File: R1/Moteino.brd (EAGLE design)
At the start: 33.3 x 23.1 mm, 21 parts, among them IC3 MCP1703CB, X1 16 MHz

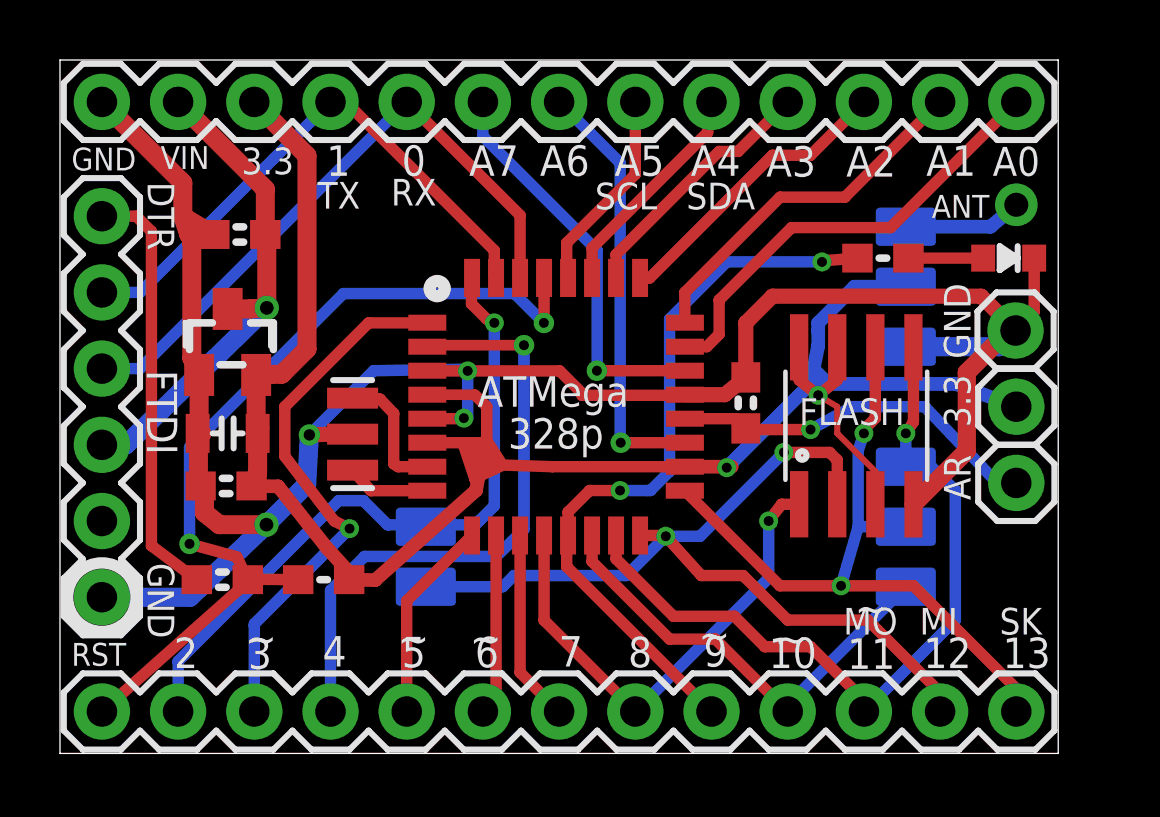
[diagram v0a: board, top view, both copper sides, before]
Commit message: R2 Update
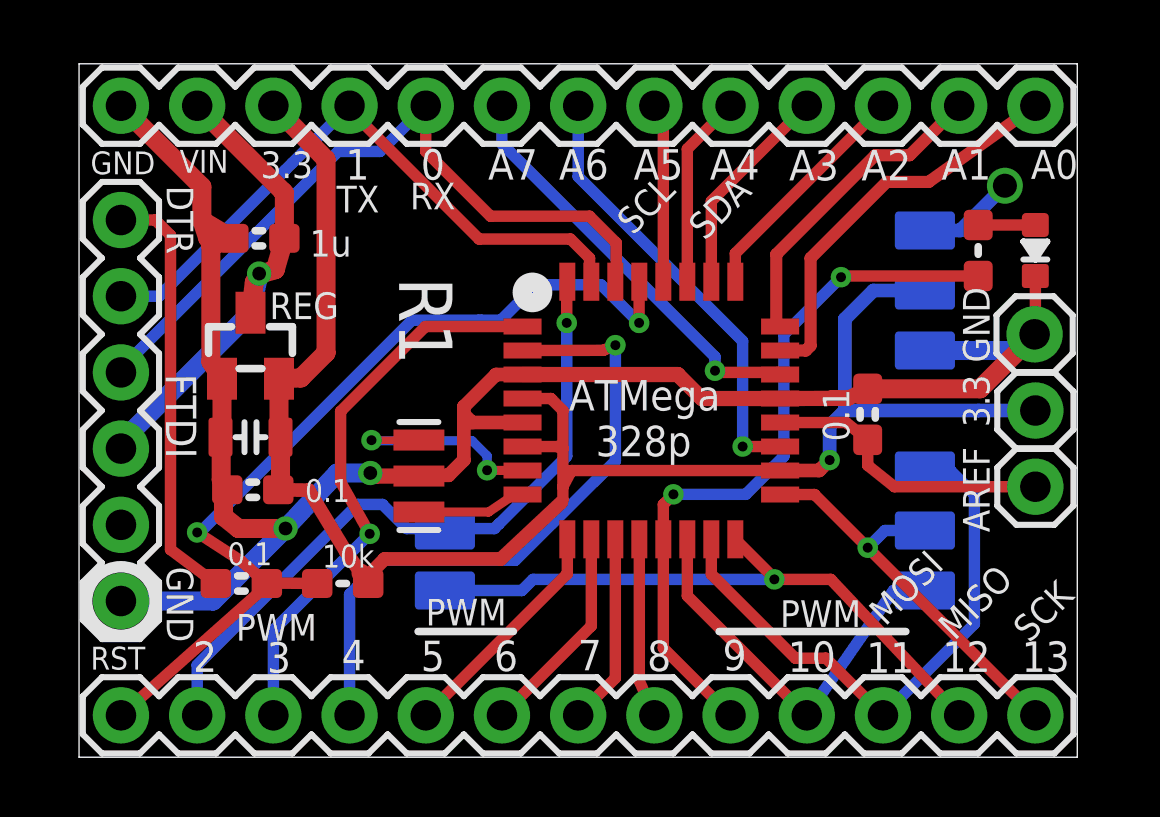
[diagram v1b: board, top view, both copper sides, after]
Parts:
- removed U$4: AT25F512BJEDEC, LowPowerLab:SO08
- moved C5 4.08 mm to (26.9, 11.3)
- moved R2 3.19 mm to (30.6, 16.8), turned to 270 degrees
- moved ATMEGA328 3.18 mm to (19.7, 11.4)
- moved X1 2.61 mm to (12.0, 9.25)
- moved U$2 0.92 mm to (32.5, 16.8), turned to 90 degrees
- moved C4 0.90 mm to (6.43, 8.79)
- moved C3 0.77 mm to (6.35, 10.5)
- moved IC3 0.77 mm to (6.35, 13.6)
- moved U$1 0.74 mm to (31.5, 18.9)
- moved + 0.65 mm to (32.5, 11.4)
- moved DIGITALSIDE 0.65 mm to (32.5, 1.27)
- moved R1 0.65 mm to (9.42, 5.66)
- moved ANALOGSIDE 0.65 mm to (32.5, 21.6)
- moved JP1 0.65 mm to (32.5, 8.89)
- moved JP2 0.65 mm to (32.5, 14.0)
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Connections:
- net D11_MOSI: no longer U$4.5_SI
- net D12_MISO: no longer U$4.2_SO
- net D13_SCK: no longer U$4.6_SCK
- net D8: no longer U$4.1_CS
- net GND: no longer U$4.4_GND
- net VCC: no longer U$4.3_WP, U$4.7_HOLD, U$4.8_VCC
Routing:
- net VCC: track 72.3 -> 57.2 mm, vias 2 -> 1
- net GND: track 78.6 -> 65.8 mm, vias 4 -> 2
- net D8: track 16.6 -> 5.97 mm, vias 1 -> 0
- net D13_SCK: track 24.4 -> 13.9 mm, vias 2 -> 1
- net D12_MISO: track 30.0 -> 21.1 mm, vias 2 -> 1
- net D11_MOSI: track 26.3 -> 19.4 mm, vias 1 -> 0
- net D0_RX: track 21.3 -> 24.4 mm
- net N$1: track 4.50 -> 7.31 mm, vias 0 -> 2
- net AREF: track 12.5 -> 9.81 mm, vias 1 -> 0
- net D1_TX: track 18.7 -> 21.2 mm
- net A2: track 9.89 -> 7.91 mm
- net A0: track 15.1 -> 13.4 mm
- net D10_SS: track 15.3 -> 13.6 mm
- net A3: track 8.61 -> 7.19 mm
- net RST: track 30.2 -> 31.6 mm
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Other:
- board text added: "IN"
- board text added: "Lowpowerlab.com"
- board text added: "MISO"
- board text added: "MOSI"
- board text added: "OUT"
- board text added: "PWM"
- board text added: "R1"
- board text added: "SCK"
- board text removed: "AR"
- board text removed: "FLASH"
- board text removed: "LowPowerLab.com"
- board text removed: "MI"
- board text removed: "MO"
- board text removed: "R2"
- board text removed: "SK"
- board text removed: "~"
